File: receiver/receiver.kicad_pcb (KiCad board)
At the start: 2 copper layers, 58.7 x 53.8 mm, 62 parts, among them J1 USB_B_Mini, J2 Conn_01x04_Pin, J3 Conn_01x04_Pin, SW1 SW_Push, SW2 SW_SPDT, U1 AMS1117-3.3, U2 STM32F303K8Tx, U3 Si590, U4 HMC356, U5 LT5517, U6 MABAES0054, U7 FT232RL, U8 AMK-2-13+, Y1 16MHz

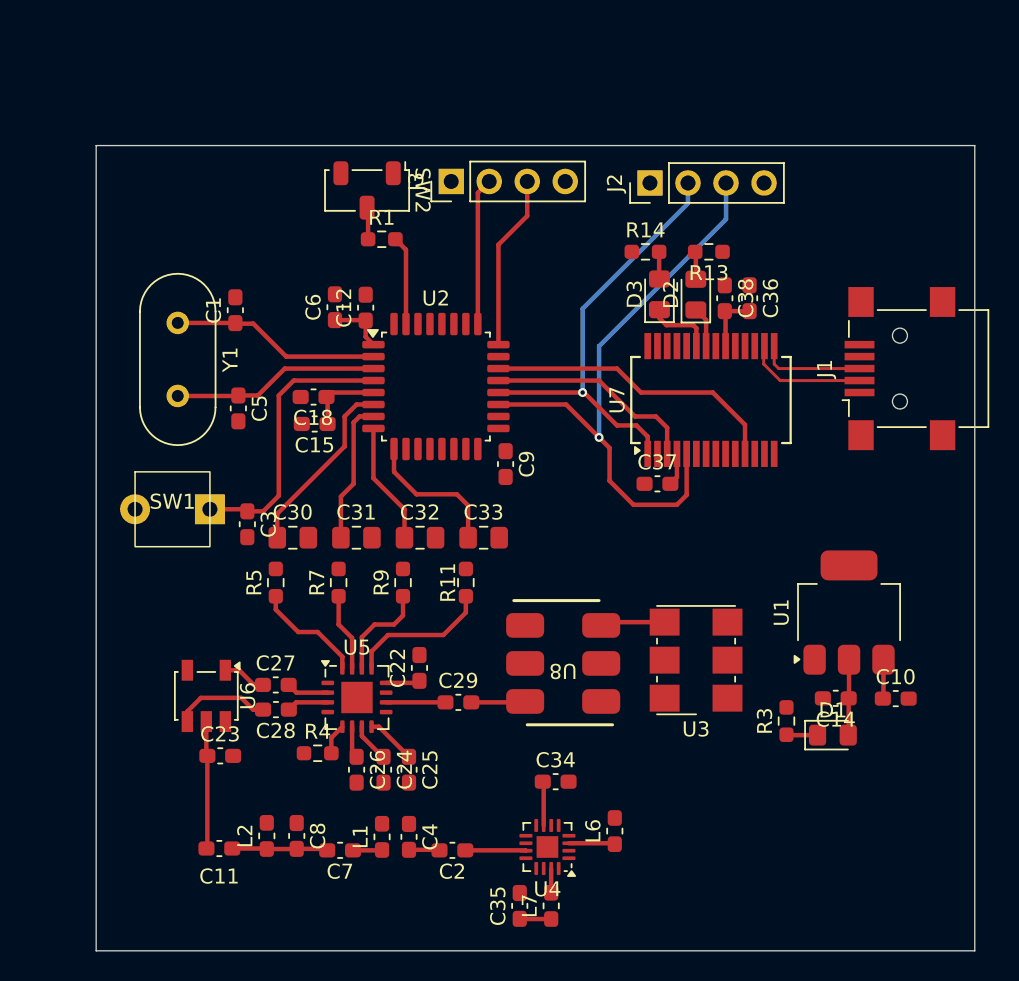
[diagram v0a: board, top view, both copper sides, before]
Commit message: Finished PCB design
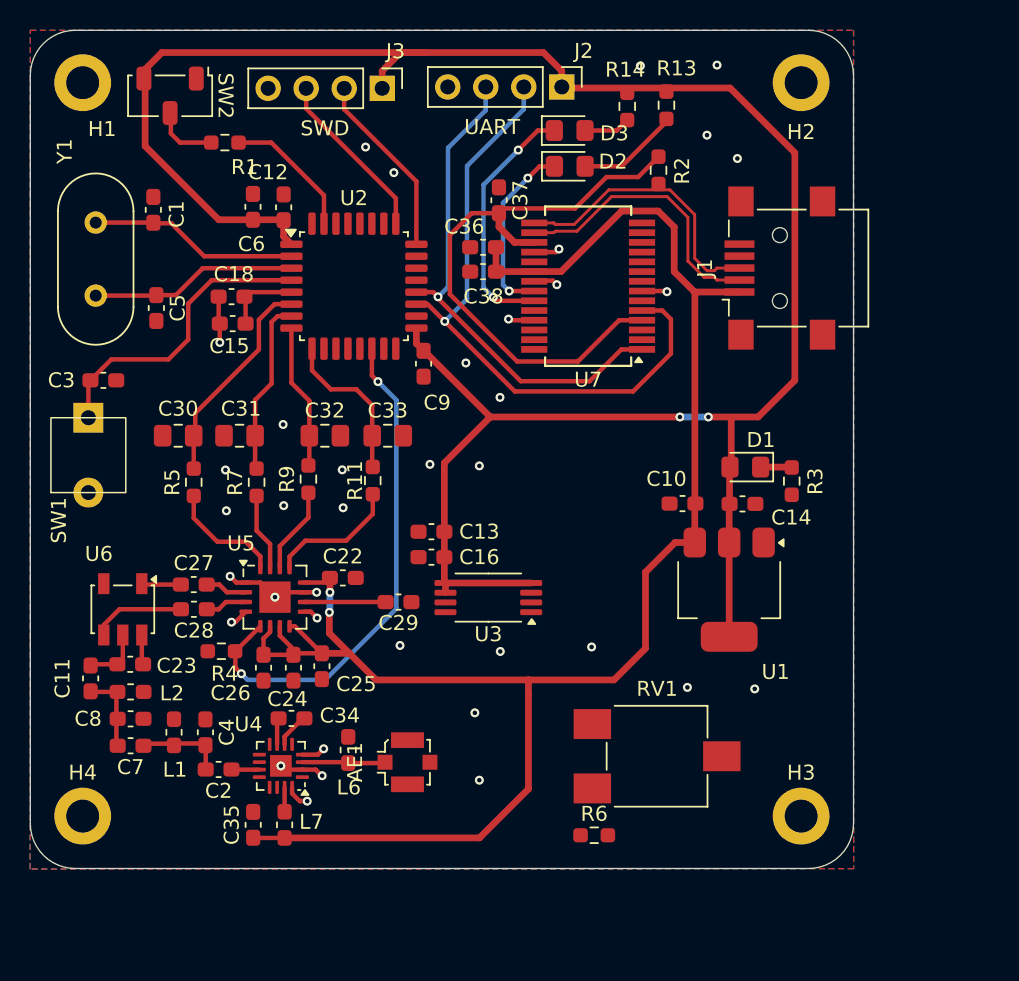
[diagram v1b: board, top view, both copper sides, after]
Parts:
- removed U8: AMK-2-13+, Communication_circuit:6-SMD-2.54
- added AE1: Antenna_Shield, Connector_Coaxial:U.FL_Molex_MCRF_73412-0110_Vertical, F.Cu at (107.2, 118.9)
- added C13: 220p, Capacitor_SMD:C_0603_1608Metric_Pad1.08x0.95mm_HandSolder, F.Cu at (108.8, 103.5)
- added C16: 220p, Capacitor_SMD:C_0603_1608Metric_Pad1.08x0.95mm_HandSolder, F.Cu at (108.8, 105.2)
- added H1: MountingHole_Pad, MountingHole:MountingHole_2.2mm_M2_DIN965_Pad, F.Cu at (85.5, 73.5)
- added H2: MountingHole_Pad, MountingHole:MountingHole_2.2mm_M2_DIN965_Pad, F.Cu at (133.5, 73.5)
- added H3: MountingHole_Pad, MountingHole:MountingHole_2.2mm_M2_DIN965_Pad, F.Cu at (133.5, 122.5)
- added H4: MountingHole_Pad, MountingHole:MountingHole_2.2mm_M2_DIN965_Pad, F.Cu at (85.5, 122.5)
- added R2: 1.5k, Resistor_SMD:R_0603_1608Metric_Pad0.98x0.95mm_HandSolder, F.Cu at (124.0, 79.4)
- added R6: 3.9k, Resistor_SMD:R_0603_1608Metric_Pad0.98x0.95mm_HandSolder, F.Cu at (119.7, 123.8)
- added RV1: R_Potentiometer, Potentiometer_SMD:Potentiometer_ACP_CA6-VSMD_Vertical, F.Cu at (123.9, 118.5)
- U3: value Si590 -> MAX2622; footprint Oscillator:Oscillator_SMD_IDT_JU6-6_7.0x5.0mm_P2.54mm -> Package_SO:TSSOP-8_4.4x3mm_P0.65mm
- moved C37 21.7 mm to (113.3, 81.4), turned to -90 degrees
- moved C10 19.3 mm to (125.6, 101.6), turned to 180 degrees
- moved D1 18.8 mm to (129.8, 99.2), turned to 180 degrees
- moved C35 18.6 mm to (96.9, 123.1)
- moved L6 18.6 mm to (103.2, 118.1)
- moved L7 18.6 mm to (99.0, 123.1)
- moved U4 18.6 mm to (98.7, 119.1)
- moved C34 18.1 mm to (99.5, 116.0)
- moved C36 18.1 mm to (112.2, 84.5), turned to 0 degrees
- moved C2 16.5 mm to (94.6, 119.4)
- moved C38 16.2 mm to (112.2, 86.1), turned to 0 degrees
- moved R3 16.0 mm to (132.9, 100.1), turned to -90 degrees
- moved C7 15.6 mm to (88.7, 117.8)
- moved L1 15.6 mm to (91.6, 116.9)
- moved C4 15.3 mm to (93.7, 116.9)
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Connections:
- net RF_ANTENNA_INPUT renamed Net-(AE1-A)
- C37 pad 2: +3V3 -> 3V3
- J2 pad 2: USART1_RX -> USART1_TX
- J2 pad 3: USART1_TX -> USART1_RX
- J3 pad 2: SWDIO -> SWCLK
- J3 pad 3: SWCLK -> SWDIO
- R13 pad 1: +5V -> +3V3
- R14 pad 1: +5V -> +3V3
- U2 pad 21: USART1_CTS -> unconnected-(U2-PA11-Pad21)
- U2 pad 22: USART1_RTS -> unconnected-(U2-PA12-Pad22)
- U3 pad 1: +3V3 -> unconnected-(U3-NC-Pad1)
- U3 pad 2: unconnected-(U3-OC-Pad2) -> Net-(U3-TUNE)
- U3 pad 4: Net-(U3-CLK_P) -> +3V3
- U3 pad 5: unconnected-(U3-CLK_N-Pad5) -> +3V3
- U7 pad 11: USART1_RTS -> unconnected-(U7-CTS-Pad11)
- U7 pad 17: +3V3 -> 3V3
- U7 pad 3: USART1_CTS -> unconnected-(U7-RTS-Pad3)
- U7 pad 4: +3V3 -> 3V3
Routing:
- net +3V3: track 11.2 -> 147.9 mm, vias 0 -> 2
- net +5V: track 19.1 -> 118.3 mm, vias 0 -> 2
- net 3V3: track 0.00 -> 39.6 mm
- net EN: track 2.08 -> 34.6 mm, vias 0 -> 2
- net GND: track 0.00 -> 29.3 mm, vias 0 -> 37
- net USART1_RTS: track 20.0 -> 0.00 mm
- net USART1_CTS: track 14.3 -> 0.00 mm
- net TX_LED: track 4.51 -> 16.9 mm, vias 0 -> 2
- net USB_D+: track 7.02 -> 18.7 mm
- net USB_D-: track 8.08 -> 18.7 mm
- net RX_LED: track 2.71 -> 12.2 mm, vias 0 -> 2
- net Net-(D2-A): track 1.85 -> 6.85 mm
- net BPF_output: track 8.59 -> 3.91 mm
- net USART1_RX: track 29.3 -> 33.8 mm
- net Net-(U3-CLK_P): track 4.33 -> 0.00 mm
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- added copper zone on B.Cu, net GND
- added copper zone on F.Cu, net GND
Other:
- board size 58.7 x 53.8 mm -> 55 x 56 mm
- board text added: "SWD"
- board text added: "UART"
